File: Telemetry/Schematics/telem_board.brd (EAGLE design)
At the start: 68.2 x 66 mm, 29 parts, among them IC1 PIC18F26K80I/SP, IC2 PTN78000WAH, IC3 ISO1050DUB, IC4 SN75LBC179D, J1 ICD, J2 CANBUS, J3 CANBUS, J4 HALLSENS, J5 TEMPSENS, J7 RADIO, Q4 20M, X1 +12V

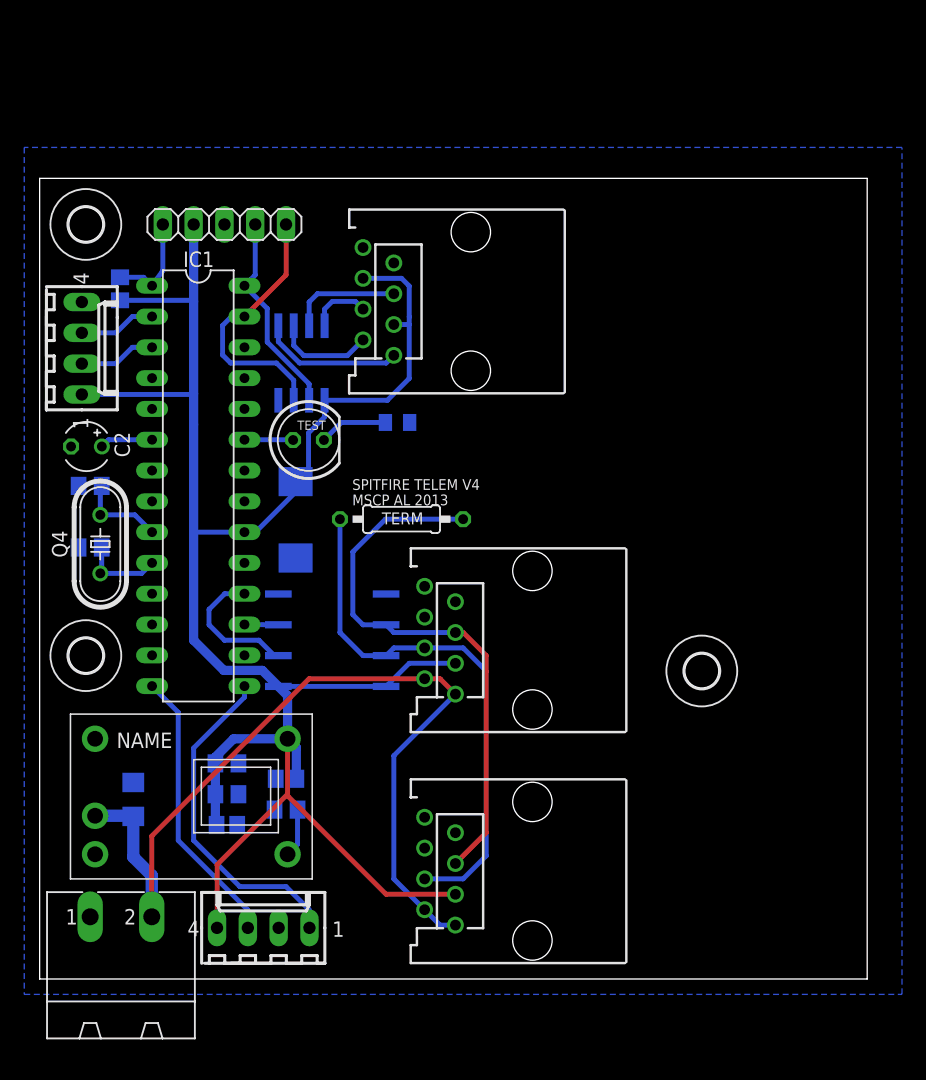
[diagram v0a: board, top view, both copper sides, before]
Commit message: v5
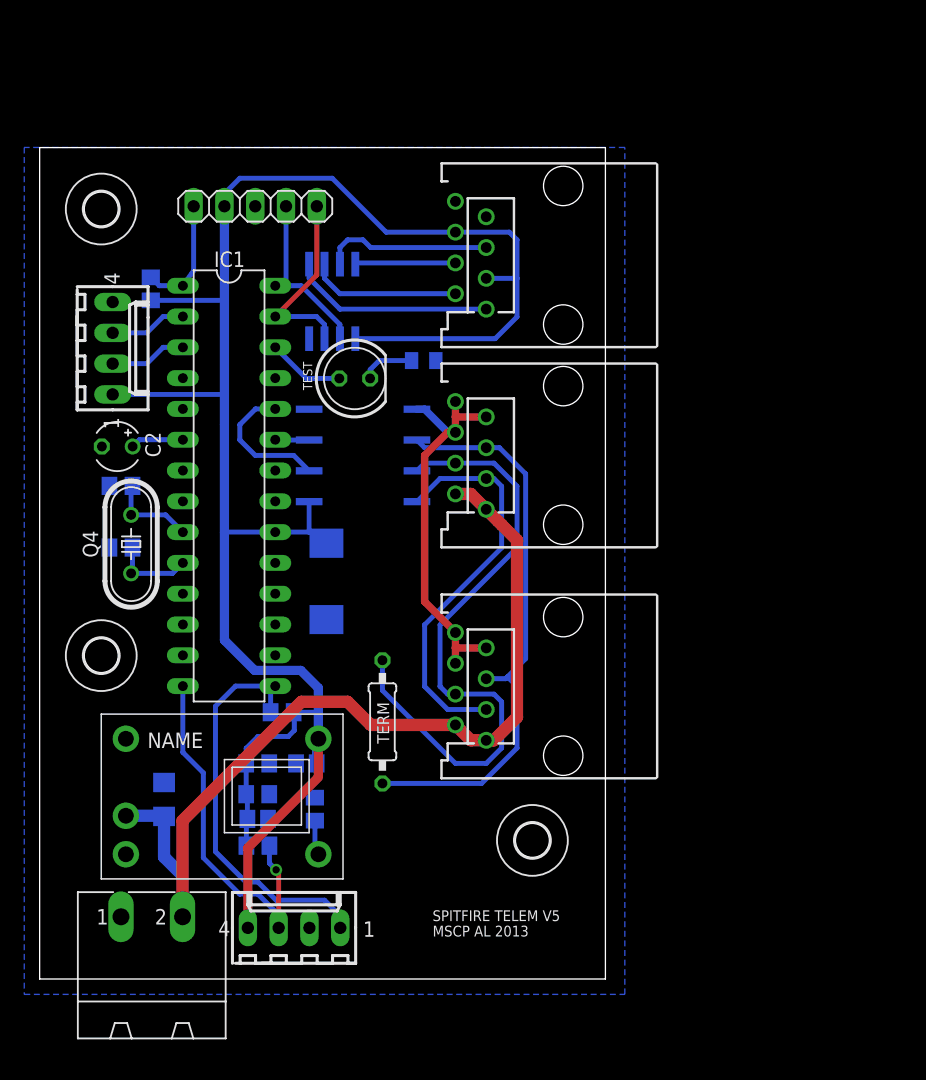
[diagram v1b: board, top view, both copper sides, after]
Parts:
- added R3, R5: (no value), eagle-ltspice:R0805
- moved H4 19.8 mm to (40.6, 11.4)
- moved TERM 16.8 mm to (28.3, 21.2), turned to 270 degrees
- moved IC3 15.5 mm to (26.7, 43.2)
- moved J2 15.5 mm to (43.2, 43.2)
- moved J3 15.5 mm to (43.2, 24.1)
- moved J7 8.52 mm to (43.2, 59.7)
- moved TEST 6.35 mm to (26.0, 49.5)
- moved IC4 5.68 mm to (24.1, 55.9)
- moved C4 5.68 mm to (23.6, 32.8)
- moved R2 5.54 mm to (31.7, 51.0)
- moved J1 2.95 mm to (17.8, 63.7)
- moved C11 2.59 mm to (18.0, 13.2)
- moved C5 2.54 mm to (18.0, 15.2)
- moved C6 2.54 mm to (18.0, 17.8)
- moved IC1 2.54 mm to (15.6, 40.7)
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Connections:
- removed net CTS: IC1.24
- removed net N$18: IC1.18, IC3.2
- removed net RTS: IC1.26
- new net CAN5V: IC3.8, J2.3, J3.3
- new net CANGND: IC3.5, J2.6, J2.7, J2.8, J3.6, J3.7, J3.8
- new net N$9: IC1.24, IC3.2
- net +5V: now also R3.1, R5.1; no longer IC3.8, J2.3, J3.3
- net GND: no longer IC3.5, J2.6, J2.7, J2.8, J3.6, J3.7, J3.8
- net N$11: now also IC1.26, TEST.A; no longer IC1.17, IC3.3
- net N$6: now also IC3.3; no longer TEST.A
- net SCL: now also R3.2
- net SDA: now also R5.2
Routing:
- net CANGND: track 0.00 -> 33.1 mm
- net CAN5V: track 0.00 -> 33.0 mm
- net N$9: track 0.00 -> 11.5 mm
- net N$18: track 11.5 -> 0.00 mm
- net CANH: track 44.4 -> 53.2 mm
- net SCL: track 23.2 -> 31.2 mm, vias 0 -> 1
- net +5V: track 169.7 -> 163.7 mm
- net TX: track 21.9 -> 16.0 mm
- net SDA: track 27.9 -> 33.4 mm
- net N$12: track 11.8 -> 16.8 mm
- net N$3: track 9.22 -> 14.0 mm
- net N$10: track 8.22 -> 12.5 mm
- net N$11: track 2.79 -> 6.35 mm
- net N$4: track 5.07 -> 8.30 mm
- net RX: track 17.1 -> 14.4 mm
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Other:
- board size 68.2 x 66 mm -> 46.7 x 68.6 mm
- board text added: "SPITFIRE TELEM V5"
- board text removed: "SPITFIRE TELEM V4"

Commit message: v6
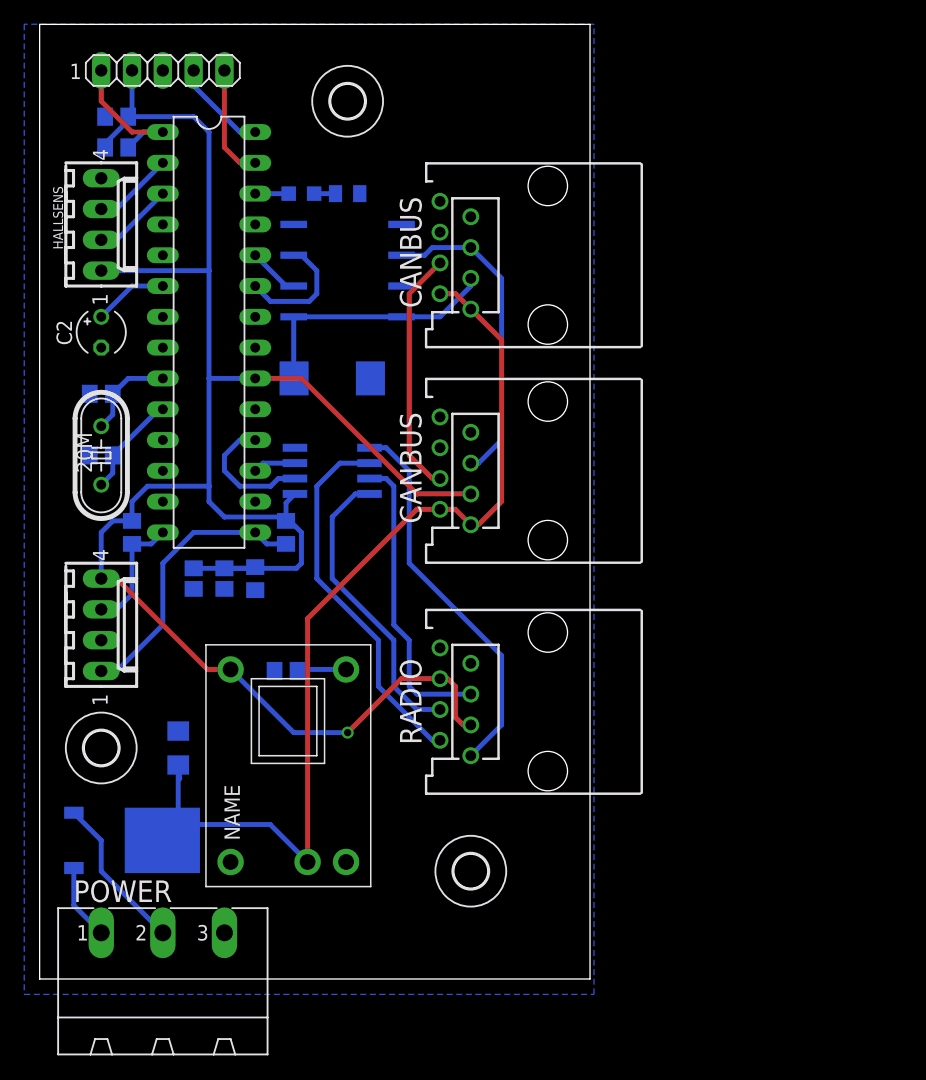
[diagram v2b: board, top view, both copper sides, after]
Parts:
- removed J1: ICD, pinhead:1X05
- removed TERM: 100, resistor:0207/10
- removed X1: +12V, con-phoenix-508:MSTBA2
- added 1: ICD, pinhead:1X05
- added DPAK: DIODE_2SCHOTTKY-DPAK, MSCP_2011_v2:DPAK
- added POWER: MSTBA3, con-phoenix-508:MSTBA3
- TEST: device led:LED5MM -> led:CHIP-LED0805
- moved C6 54.6 mm to (6.35, 71.1), turned to 180 degrees
- moved J7 36.9 mm to (41.9, 22.9)
- moved J5 29.6 mm to (5.08, 29.2), turned to 270 degrees
- moved R3 27.8 mm to (7.62, 36.8), turned to 270 degrees
- moved H3 22.2 mm to (25.4, 72.4)
- moved C11 20.0 mm to (15.2, 33.0), turned to 270 degrees
- moved C12 17.9 mm to (12.7, 33.0), turned to 270 degrees
- moved J3 17.8 mm to (41.9, 41.9)
- moved C5 17.8 mm to (17.8, 33.0), turned to 270 degrees
- moved C4 16.7 mm to (24.1, 49.5), turned to 180 degrees
- moved J2 16.6 mm to (41.9, 59.7)
- moved TEST 15.9 mm to (21.6, 64.8), flipped to the bottom, turned to 90 degrees
- moved IC3 15.3 mm to (25.4, 58.4)
- moved R2 15.1 mm to (25.4, 64.8)
- moved R5 14.8 mm to (20.3, 36.8), turned to 270 degrees
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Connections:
- net N$11 renamed STATUS
- removed net CAN5V: IC3.8, J2.3, J3.3
- removed net CANGND: IC3.5, J2.6, J2.7, J2.8, J3.6, J3.7, J3.8
- new net N$13: DPAK.1, POWER.1
- new net N$14: DPAK.2, POWER.2
- new net N$15: 1.4, IC1.28
- new net N$16: 1.5, IC1.27
- net +12V: now also DPAK.3; no longer X1.2
- net +5V: now also 1.2, IC3.8, J2.3, J3.3; no longer J1.2
- net CANH: no longer TERM.1
- net CANL: no longer TERM.2
- net GND: now also 1.3, IC3.5, J2.6, J2.7, J2.8, J3.6, J3.7, J3.8, POWER.3; no longer J1.3, X1.1
- net N$20: now also 1.1; no longer J1.1
- net N$7: now also TEST.C; no longer TEST.K
- net RX: now also IC1.18; no longer IC1.28, J1.4
- net TX: now also IC1.17; no longer IC1.27, J1.5
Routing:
- net CANGND: track 33.1 -> 0.00 mm
- net CAN5V: track 33.0 -> 0.00 mm
- net CANH: track 53.2 -> 24.2 mm
- net CANL: track 47.8 -> 26.2 mm
- net +5V: track 163.7 -> 185.1 mm, vias 0 -> 1
- net SCL: track 31.2 -> 10.1 mm, vias 1 -> 0
- net N$10: track 12.5 -> 30.7 mm
- net N$4: track 8.30 -> 24.5 mm
- net N$12: track 16.8 -> 31.8 mm
- net N$14: track 0.00 -> 12.9 mm
- net TX: track 16.0 -> 3.54 mm
- net N$3: track 14.0 -> 24.6 mm
- net SDA: track 33.4 -> 23.3 mm
- net N$16: track 0.00 -> 9.42 mm
- net N$15: track 0.00 -> 7.93 mm
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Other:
- board size 46.7 x 68.6 mm -> 45.4 x 78.7 mm
- board text added: "MSCP AL 2014 TELEM V6"
- board text removed: "MSCP AL 2013"
- board text removed: "SPITFIRE TELEM V5"
